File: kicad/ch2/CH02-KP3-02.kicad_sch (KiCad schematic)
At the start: 5 parts

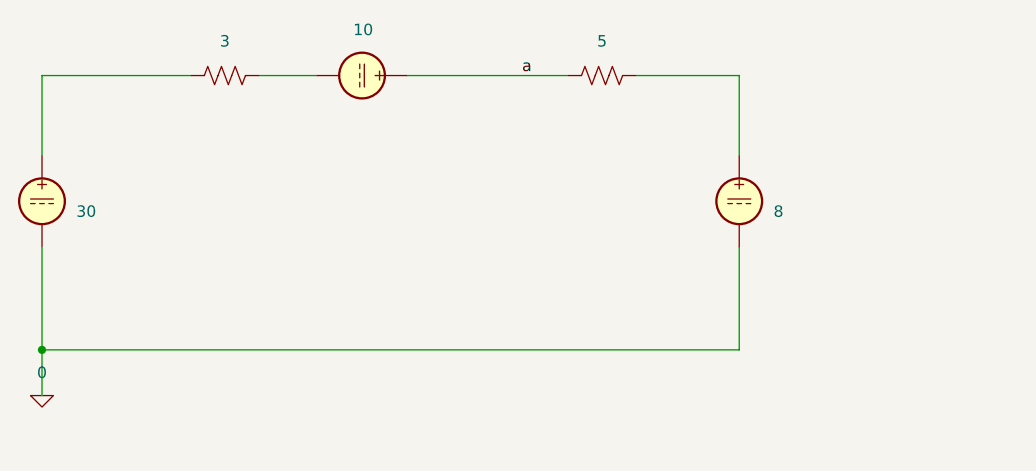
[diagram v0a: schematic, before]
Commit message: regular
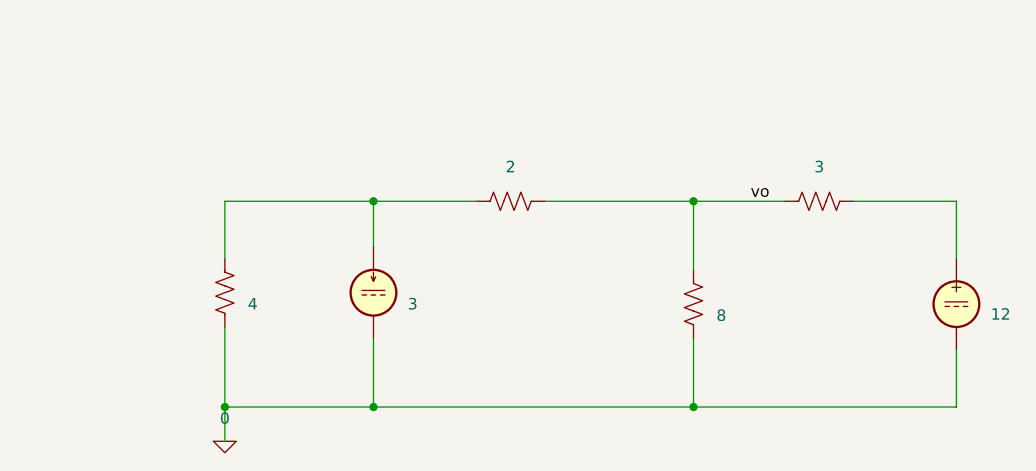
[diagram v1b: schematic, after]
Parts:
- removed R4: 3, symbol Device:R_US
- removed R5: 5, symbol Device:R_US
- removed V3: 30, symbol Simulation_SPICE:VDC
- removed V4: 10, symbol Simulation_SPICE:VDC
- removed V5: 8, symbol Simulation_SPICE:VDC
- added I1: 3, symbol Simulation_SPICE:IDC
- added R6: 4, symbol Device:R_US
- added R7: 2, symbol Device:R_US
- added R8: 3, symbol Device:R_US
- added R9: 8, symbol Device:R_US
- added V6: 12, symbol Simulation_SPICE:VDC
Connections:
- net 0: now also I1.2, R6.2, R9.2, V6.2
- new net: I1.1, R6.1, R7.1
- new net: R8.2, V6.1
- new net vo: R7.2, R8.1, R9.1
